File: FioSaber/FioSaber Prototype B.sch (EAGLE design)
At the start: 19 parts, among them P1 WIICHUCK, T1 2N2222

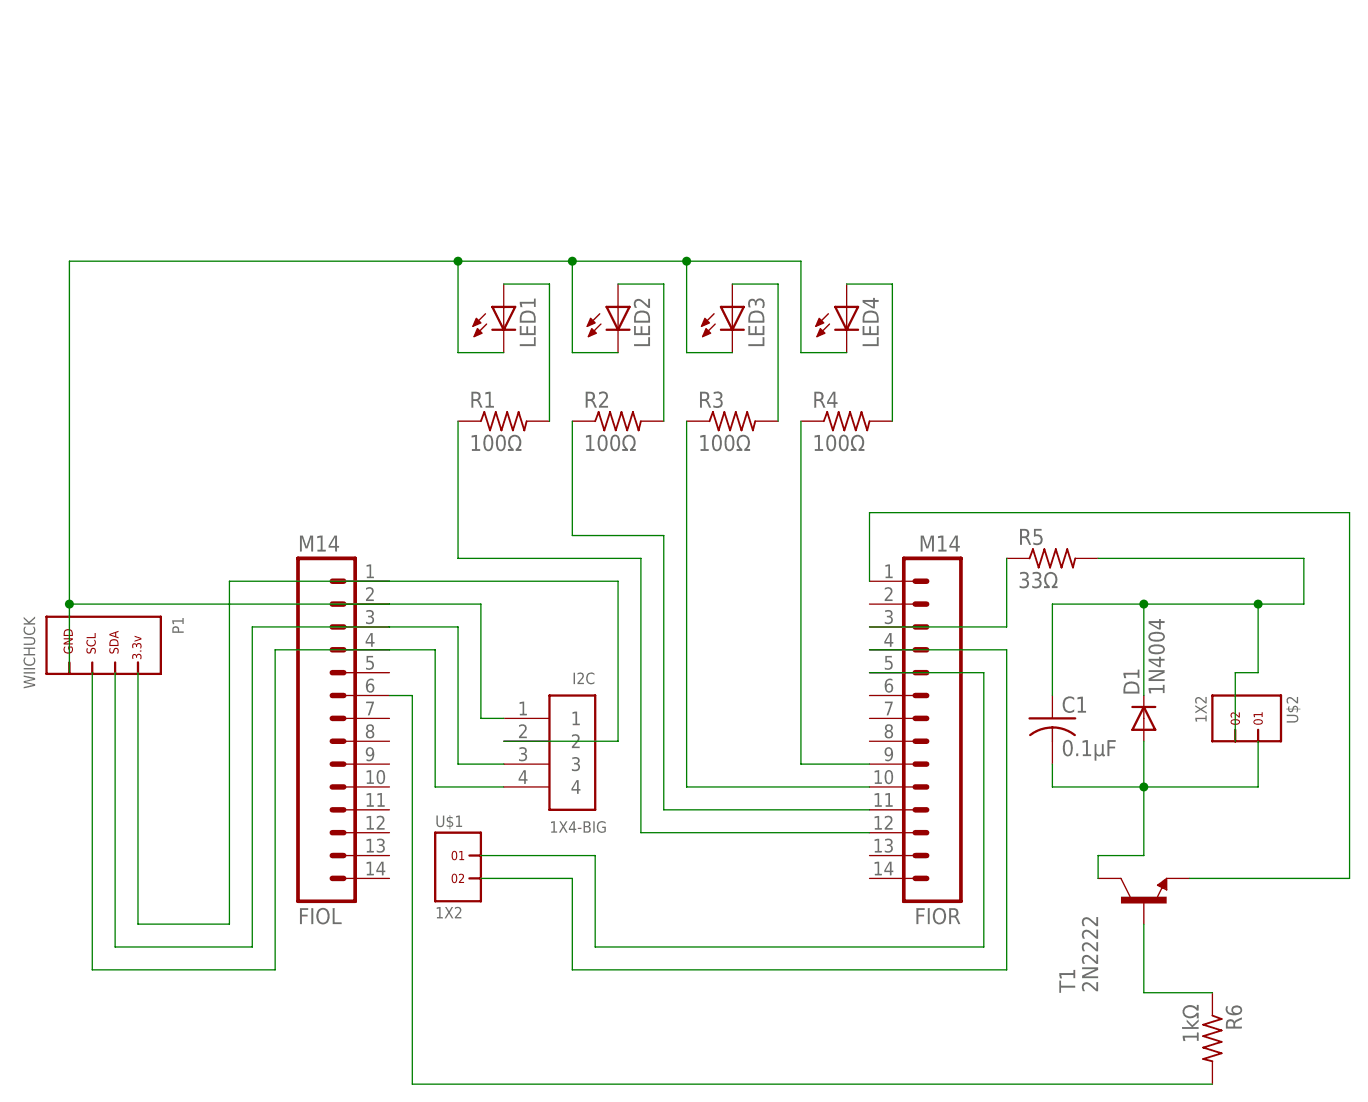
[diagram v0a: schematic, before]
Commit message: prototype b
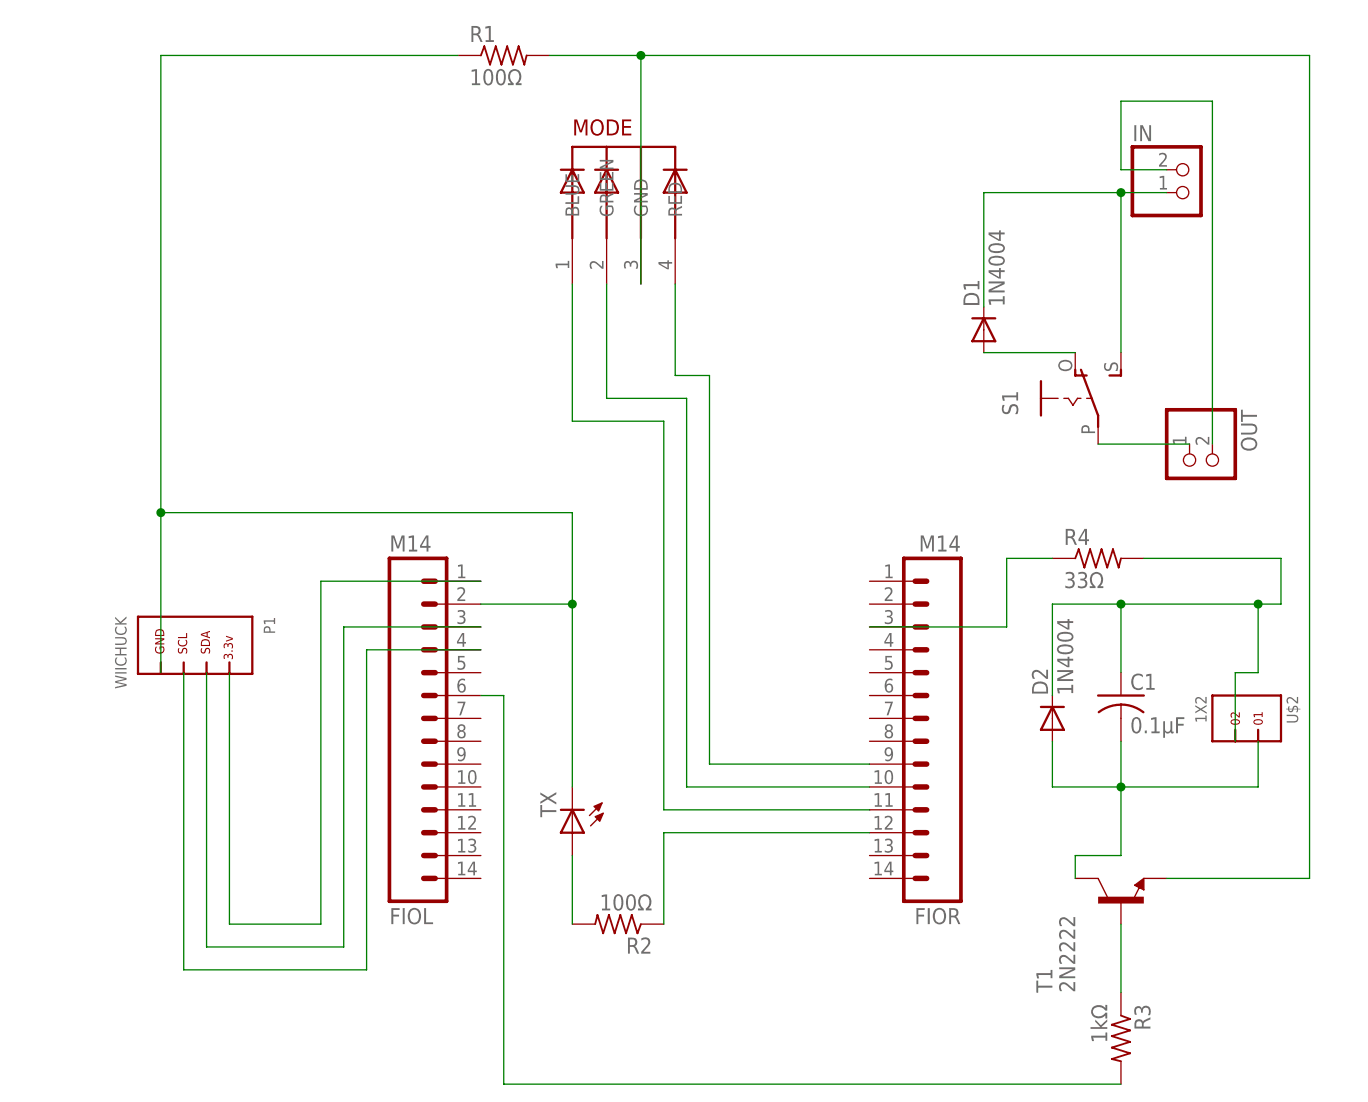
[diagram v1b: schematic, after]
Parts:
- removed I2C: 1X4-BIG, adafruit:1X4-BIG
- removed LED1, LED2, LED3, LED4: (no value), adafruit:LED3MM
- removed R5: 33Ω, adafruit:R-US_0207/10
- removed R6: 1kΩ, adafruit:R-US_0207/10
- removed U$1: 1X2, headers(.1in):1X2
- added D2: 1N4004, adafruit:1N4004
- added IN, OUT: (no value), adafruit:JST_2PIN-SMT-RA
- added MODE: 5MMRGBLED, adafruit:5MMRGBLED
- added S1: (no value), adafruit:EG1218S
- added TX: (no value), adafruit:LED3MM
- R3: value 100Ω -> 1kΩ
- R4: value 100Ω -> 33Ω
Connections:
- removed net N$14: FIOR.4, U$1.2
- removed net N$15: FIOR.5, U$1.1
- new net N$25: R2.2, TX.A
- net N$1: no longer I2C.2
- net N$10: now also OUT.2, S1.P; no longer LED2.A, R2.2
- net N$11: now also IN.1, OUT.1; no longer LED3.A, R3.2
- net N$12: now also FIOR.3, R4.1; no longer LED4.A, R4.2
- net N$13: now also MODE.GND, R1.2, T1.E; no longer FIOL.2, I2C.1, LED1.C, LED2.C, LED3.C, LED4.C, P1.GND
- net N$16: now also R3.2; no longer R6.2
- net N$17: now also FIOR.12, R2.1; no longer FIOR.1, T1.E
- net N$18: now also R3.1; no longer R6.1
- net N$19: now also D2.A; no longer D1.A
- net N$2: now also D1.C, IN.2, S1.S; no longer FIOR.3, R5.1
- net N$20: now also D2.C, R4.2; no longer D1.C, R5.2
- net N$3: no longer I2C.3
- net N$4: no longer I2C.4
- net N$5: now also D1.A, S1.O; no longer FIOR.12, R1.1
- net N$6: now also MODE.BLUE; no longer R2.1
- net N$7: now also MODE.GREEN; no longer R3.1
- net N$8: now also MODE.RED; no longer R4.1
- net N$9: now also FIOL.2, P1.GND, R1.1, TX.C; no longer LED1.A, R1.2
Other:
- moved on the sheet: C1, D1, FIOL, P1, R1, R2, R3, R4, T1
